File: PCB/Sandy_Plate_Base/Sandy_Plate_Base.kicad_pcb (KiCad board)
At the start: 2 copper layers, 285 x 84.3 mm, 1 part

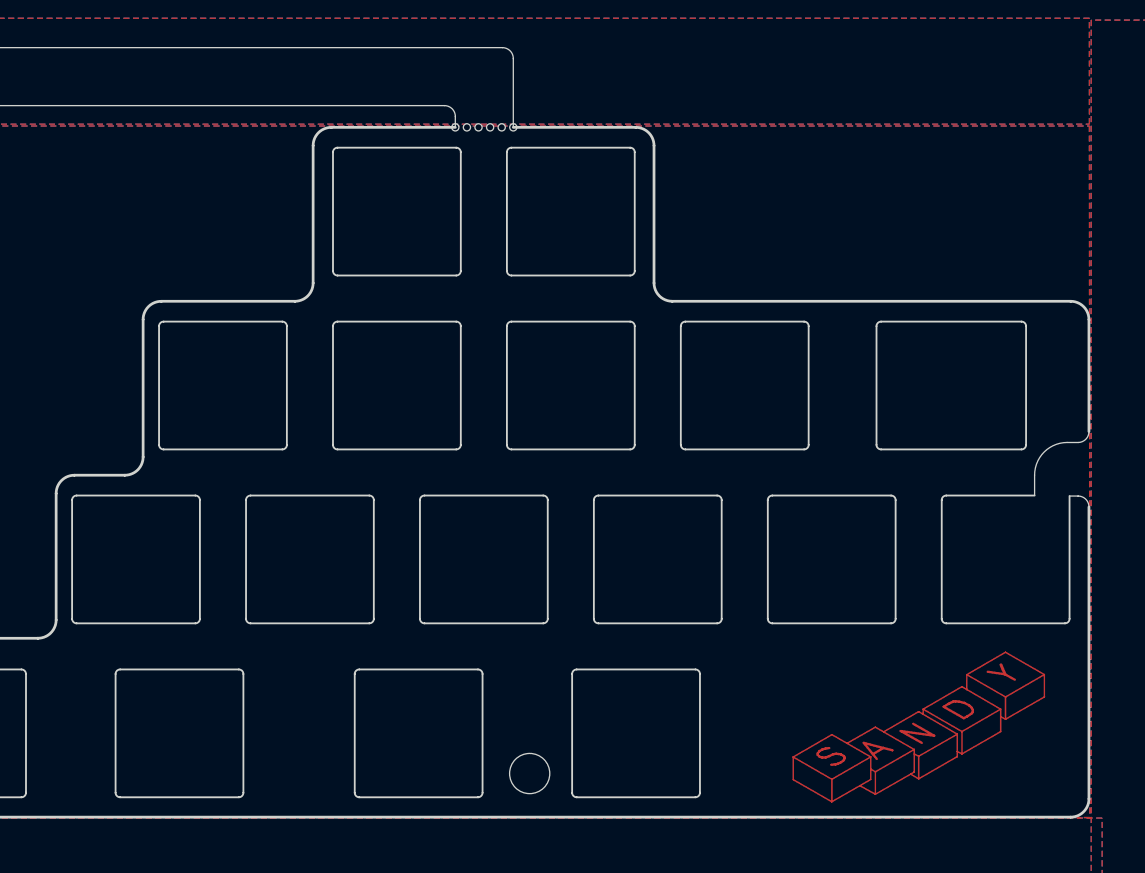
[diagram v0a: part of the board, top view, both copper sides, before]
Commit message: 更新：ビルドナンバー　→　DN0030
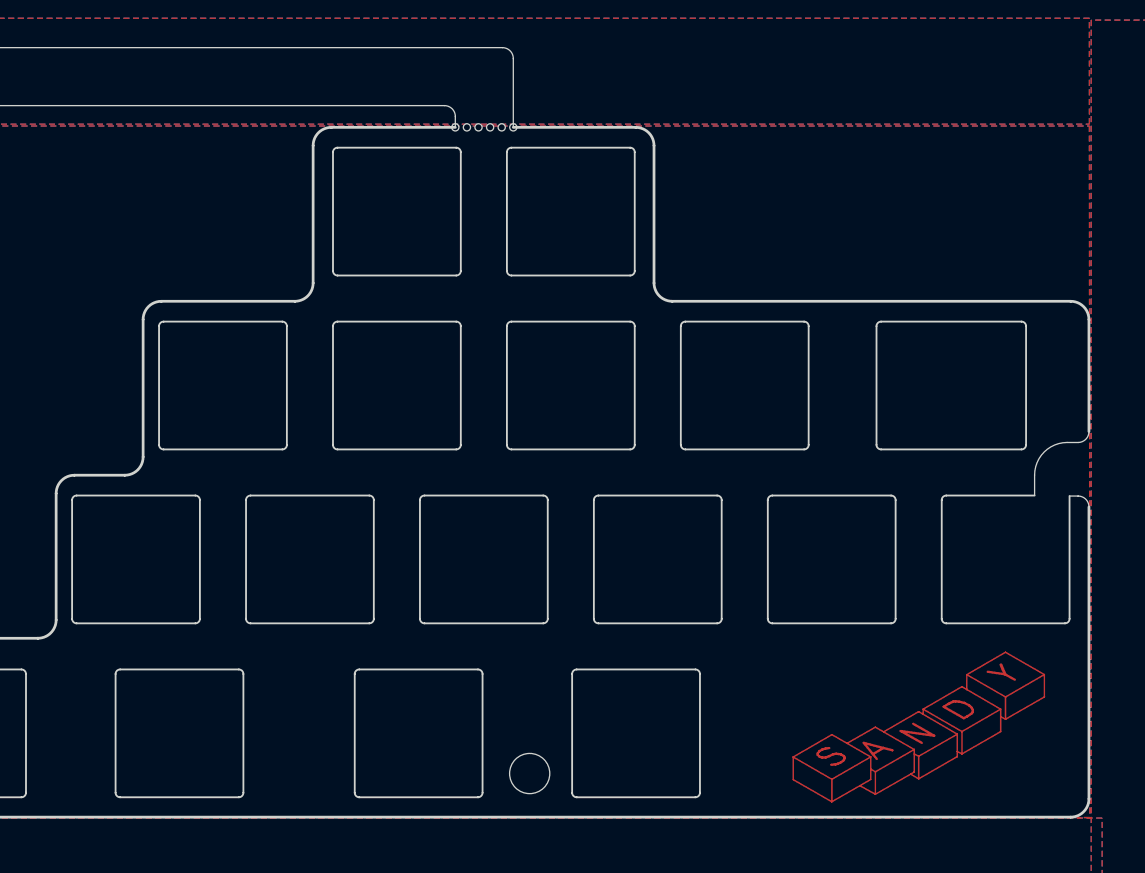
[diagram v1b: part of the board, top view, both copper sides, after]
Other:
- board text added: "#Sandy_kbd DN0030, Plate for Base by @jpskenn"
- board text removed: "#Sandy_kbd DN0020, Plate for Base by @jpskenn"
